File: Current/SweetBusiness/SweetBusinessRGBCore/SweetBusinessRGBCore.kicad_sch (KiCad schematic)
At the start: 266 parts, among them J1 Bridge

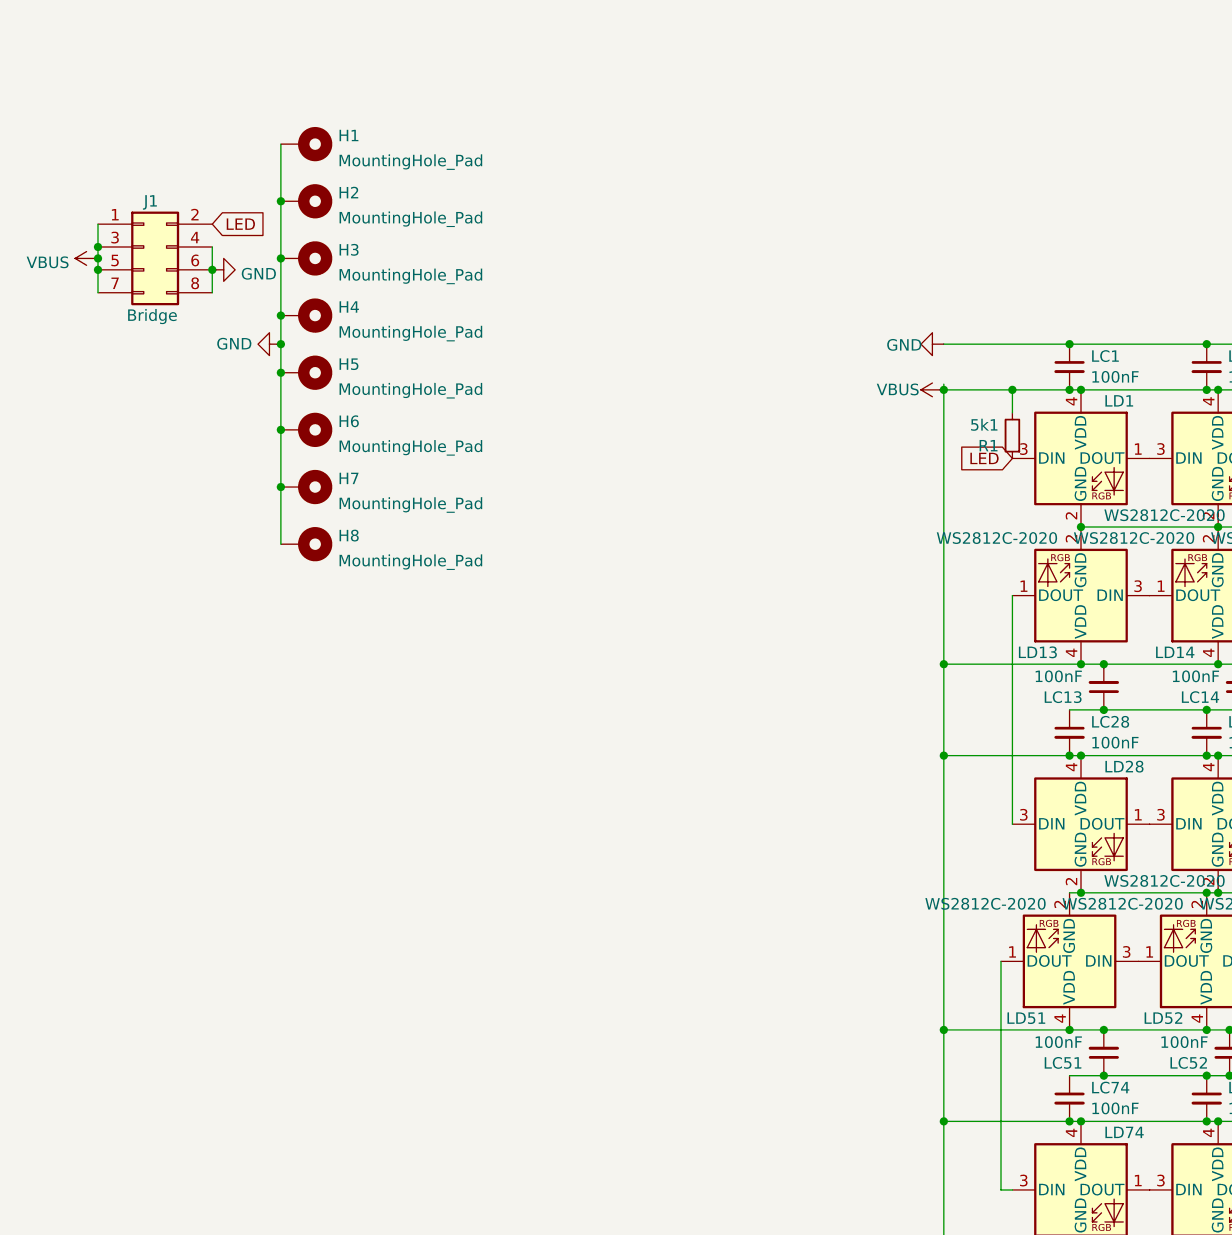
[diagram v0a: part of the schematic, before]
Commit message: oh my god just stop
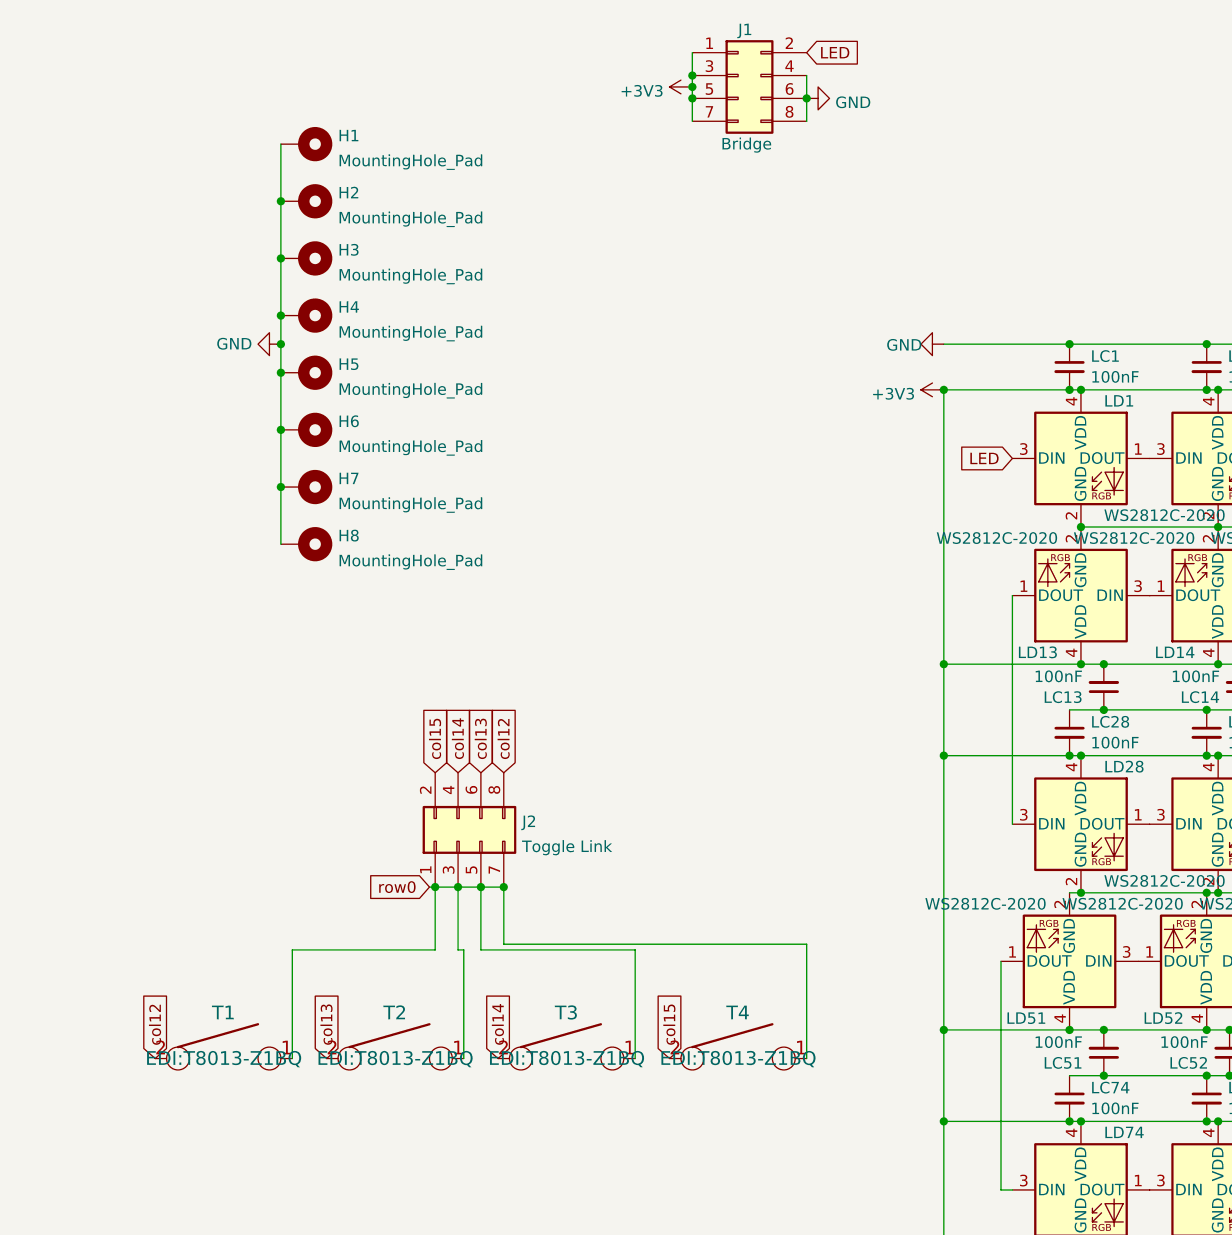
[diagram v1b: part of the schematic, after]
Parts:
- removed R1: 5k1, EDI:Passive_0402_1005Metric, symbol Device:R_Small
- added J2: Toggle Link, Connector_PinHeader_2.54mm:PinHeader_2x04_P2.54mm_Vertical, symbol Connector_Generic:Conn_02x04_Odd_Even
- added T1, T2, T3, T4: Keyswitch, EDI:T8013-Z1BQ, symbol EDI:Keyswitch
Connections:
- net VBUS renamed +3V3
- new net col12: J2.8 (Pin_8), T1.2
- new net col13: J2.6 (Pin_6), T2.2
- new net col14: J2.4 (Pin_4), T3.2
- new net col15: J2.2 (Pin_2), T4.2
- new net row0: J2.1 (Pin_1), J2.3 (Pin_3), J2.5 (Pin_5), J2.7 (Pin_7), T1.1, T2.1, T3.1, T4.1
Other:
- moved on the sheet: J1
